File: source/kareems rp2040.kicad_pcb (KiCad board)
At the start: 2 copper layers, 29 x 57 mm, 38 parts, among them J1 USB_C_Receptacle_USB2.0_14P, J2 Conn_01x20, J3 Conn_01x20, J4 Conn_01x03, SW1 SW_Push, U1 RP2040, U2 W25Q16JVSS, U4 MCP1700x-330xxTT, Y1 12MHz

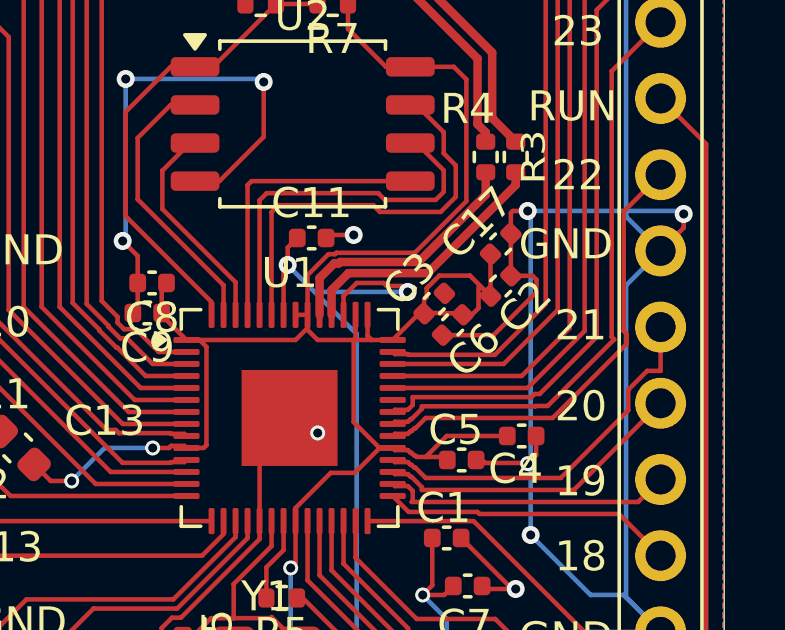
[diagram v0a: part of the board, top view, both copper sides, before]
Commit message: e
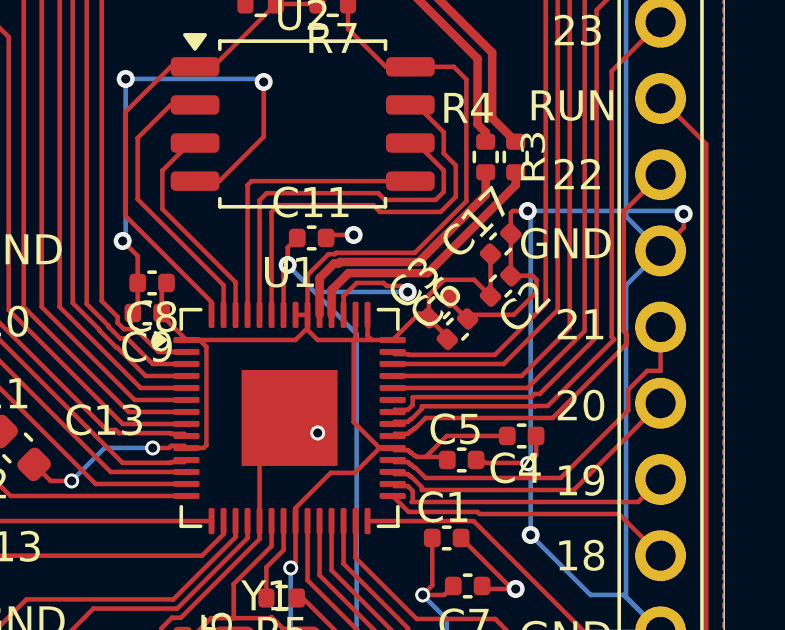
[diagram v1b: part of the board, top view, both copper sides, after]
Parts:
- moved C6 0.21 mm to (218.9, 100.3), turned to 45 degrees
- moved C3 0.21 mm to (218.2, 99.6)
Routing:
- net +3.3V: track 145.2 -> 143.3 mm
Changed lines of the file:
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@@
 	(footprint "Capacitor_SMD:C_0402_1005Metric"
 		(layer "F.Cu")
-		(at 218.7 100.2 -135)
+		(at 218.860589 100.339411 45)
 		(descr "Capacitor SMD 0402 (1005 Metric), square (rectangular) end terminal, IPC-7351 nominal, (Body size source: IPC-SM-782 page 76, https://www.pcb-3d.com/wordpress/wp-content/uploads/ipc-sm-782a_amendment_1_and_2.pdf), generated with kicad-footprint-generator")
 		(tags "capacitor")
@@
 		(attr smd)
 		(fp_line
-			(start -0.107836 0.36)
-			(end 0.107836 0.36)
+			(start -0.107836 -0.36)
+			(end 0.107836 -0.36)
 			(stroke
 				(width 0.12)
@@
 		)
 		(fp_line
-			(start -0.107836 -0.36)
-			(end 0.107836 -0.36)
+			(start -0.107836 0.36)
+			(end 0.107836 0.36)
 			(stroke
 				(width 0.12)
@@
 		)
 		(pad "1" smd roundrect
-			(at -0.48 0 225)
+			(at -0.48 0 45)
 			(size 0.56 0.62)
 			(layers "F.Cu" "F.Mask" "F.Paste")
@@
 		)
 		(pad "2" smd roundrect
-			(at 0.48 0 225)
+			(at 0.48 0 45)
 			(size 0.56 0.62)
 			(layers "F.Cu" "F.Mask" "F.Paste")
@@
 	(footprint "Capacitor_SMD:C_0402_1005Metric"
 		(layer "F.Cu")
-		(at 218.085786 99.485786 45)
+		(at 218.246375 99.625197 45)
 		(descr "Capacitor SMD 0402 (1005 Metric), square (rectangular) end terminal, IPC-7351 nominal, (Body size source: IPC-SM-782 page 76, https://www.pcb-3d.com/wordpress/wp-content/uploads/ipc-sm-782a_amendment_1_and_2.pdf), generated with kicad-footprint-generator")
 		(tags "capacitor")
@@
 	)
 	(segment
-		(start 220.060589 100.539411)
-		(end 221.4942 99.1058)
+		(start 211.4 110.85)
+		(end 213.1 112.55)
 		(width 0.1524)
 		(layer "F.Cu")
@@
 	)
 	(segment
-		(start 211.4 110.85)
-		(end 213.1 112.55)
+		(start 221.4942 98.6942)
+		(end 221.360589 98.560589)
 		(width 0.1524)
 		(layer "F.Cu")
@@
 	)
 	(segment
+		(start 219.039411 99.860589)
+		(end 220.739411 99.860589)
+		(width 0.1524)
+		(layer "F.Cu")
+		(net 1)
+	)
+	(segment
 		(start 212.2625 107.3375)
 		(end 209.641 109.959)
@@
 	)
 	(segment
-		(start 220.8 109)
-		(end 220.68 109)
+		(start 218.425197 99.146375)
+		(end 218.425197 99.246375)
 		(width 0.1524)
 		(layer "F.Cu")
@@
 	)
 	(segment
-		(start 218.360589 100.539411)
-		(end 220.060589 100.539411)
+		(start 220.8 109)
+		(end 220.68 109)
 		(width 0.1524)
 		(layer "F.Cu")
@@
 	)
 	(segment
+		(start 218.425197 99.246375)
+		(end 219.039411 99.860589)
+		(width 0.1524)
+		(layer "F.Cu")
+		(net 1)
+	)
+	(segment
 		(start 199.7904 101.0904)
 		(end 200.4304 101.7304)
@@
 	)
 	(segment
-		(start 221.4942 99.1058)
-		(end 221.4942 98.6942)
+		(start 216.8375 81.2375)
+		(end 215.325 79.725)
 		(width 0.1524)
 		(layer "F.Cu")
@@
 	)
 	(segment
-		(start 216.8375 81.2375)
-		(end 215.325 79.725)
+		(start 221.360589 98.560589)
+		(end 220.639411 98.560589)
 		(width 0.1524)
 		(layer "F.Cu")
@@
 	)
 	(segment
+		(start 220.739411 99.860589)
+		(end 221.4942 99.1058)
+		(width 0.1524)
+		(layer "F.Cu")
+		(net 1)
+	)
+	(segment
 		(start 210.35 110.85)
 		(end 209.7 111.5)
@@
 	)
 	(segment
-		(start 221.4942 98.6942)
-		(end 221.360589 98.560589)
+		(start 219.039411 99.860589)
+		(end 219.339411 99.860589)
 		(width 0.1524)
 		(layer "F.Cu")
@@
 	)
 	(segment
-		(start 221.360589 98.560589)
-		(end 220.639411 98.560589)
+		(start 221.4942 99.1058)
+		(end 221.4942 98.6942)
 		(width 0.1524)
 		(layer "F.Cu")
@@
 	)
 	(segment
-		(start 219.560589 99.639411)
-		(end 219.560589 98.939411)
-		(width 0.1524)
-		(layer "F.Cu")
-		(net 2)
-	)
-	(segment
 		(start 209.825 100.7)
 		(end 210.2625 100.7)
@@
 	)
 	(segment
-		(start 217.83365 98.974812)
-		(end 218.253634 98.554828)
-		(width 0.1524)
-		(layer "F.Cu")
-		(net 2)
-	)
-	(segment
-		(start 217.771572 99.8)
-		(end 218.257164 99.8)
-		(width 0.1524)
-		(layer "F.Cu")
-		(net 2)
-	)
-	(segment
 		(start 217.8 104.6)
 		(end 218.5 103.9)
@@
 	)
 	(segment
-		(start 218.257164 99.8)
-		(end 218.266486 99.809322)
-		(width 0.1524)
-		(layer "F.Cu")
-		(net 2)
-	)
-	(segment
 		(start 226.781 66.099)
 		(end 224.601 66.099)
@@
 	)
 	(segment
-		(start 218.988144 99.809322)
-		(end 219.039411 99.860589)
-		(width 0.1524)
-		(layer "F.Cu")
-		(net 2)
-	)
-	(segment
 		(start 213.4625 108.1375)
 		(end 213.3 108.3)
@@
 	)
 	(segment
-		(start 219.276006 98.554828)
-		(end 219.960589 99.239411)
-		(width 0.1524)
-		(layer "F.Cu")
-		(net 2)
-	)
-	(segment
 		(start 213.8625 100.3)
 		(end 213.4625 100.7)
@@
 	)
 	(segment
-		(start 218.5 103.9)
-		(end 220.52 103.9)
-		(width 0.1524)
-		(layer "F.Cu")
-		(net 2)
-	)
-	(segment
-		(start 213.4625 106.7375)
-		(end 213.4625 108.1375)
+		(start 218.360589 100.539411)
+		(end 218.360589 100.439411)
 		(width 0.1524)
 		(layer "F.Cu")
@@
 	)
 	(segment
-		(start 217.2875 91.595)
-		(end 216.475001 91.595)
+		(start 218.414223 98.694239)
+		(end 219.415417 98.694239)
 		(width 0.1524)
 		(layer "F.Cu")
@@
 	)
 	(segment
-		(start 219.58 71.12)
-		(end 218.28 71.12)
+		(start 218.5 103.9)
+		(end 220.52 103.9)
 		(width 0.1524)
 		(layer "F.Cu")
@@
 	)
 	(segment
-		(start 217.746375 99.825197)
-		(end 217.746375 99.353625)
+		(start 213.4625 106.7375)
+		(end 213.4625 108.1375)
 		(width 0.1524)
 		(layer "F.Cu")
@@
 	)
 	(segment
-		(start 217.746375 99.353625)
-		(end 217.83365 99.26635)
+		(start 217.2875 91.595)
+		(end 216.475001 91.595)
 		(width 0.1524)
 		(layer "F.Cu")
@@
 	)
 	(segment
-		(start 218.253634 98.554828)
-		(end 219.276006 98.554828)
+		(start 219.58 71.12)
+		(end 218.28 71.12)
 		(width 0.1524)
 		(layer "F.Cu")
@@
 	)
 	(segment
-		(start 217.83365 99.26635)
-		(end 217.83365 98.974812)
+		(start 210.2625 100.7)
+		(end 210.4921 100.9296)
 		(width 0.1524)
 		(layer "F.Cu")
@@
 	)
 	(segment
-		(start 210.2625 100.7)
-		(end 210.4921 100.9296)
+		(start 213.8625 100.364116)
+		(end 214.198384 100.7)
 		(width 0.1524)
 		(layer "F.Cu")
@@
 	)
 	(segment
-		(start 213.8625 100.364116)
-		(end 214.198384 100.7)
+		(start 219.415417 98.694239)
+		(end 219.960589 99.239411)
 		(width 0.1524)
 		(layer "F.Cu")
@@
 	)
 	(segment
+		(start 218.360589 100.439411)
+		(end 217.746375 99.825197)
+		(width 0.1524)
+		(layer "F.Cu")
+		(net 2)
+	)
+	(segment
 		(start 213.4625 99.8625)
 		(end 213.8625 99.8625)
@@
 	)
 	(segment
-		(start 215.21 87.529596)
-		(end 215.21 89.5)
+		(start 217.906964 99.201498)
+		(end 218.414223 98.694239)
 		(width 0.1524)
 		(layer "F.Cu")
@@
 	)
 	(segment
-		(start 207.9 79.047583)
-		(end 209.5625 80.710083)
+		(start 217.906964 99.964608)
+		(end 217.906964 99.201498)
 		(width 0.1524)
 		(layer "F.Cu")
@@
 	)
 	(segment
-		(start 219.339411 99.860589)
-		(end 219.560589 99.639411)
+		(start 215.21 87.529596)
+		(end 215.21 89.5)
+		(width 0.1524)
+		(layer "F.Cu")
+		(net 2)
+	)
+	(segment
+		(start 207.9 79.047583)
+		(end 209.5625 80.710083)
 		(width 0.1524)
 		(layer "F.Cu")
@@
 	)
 	(segment
-		(start 218.266486 99.809322)
-		(end 218.988144 99.809322)
-		(width 0.1524)
-		(layer "F.Cu")
-		(net 2)
-	)
-	(segment
 		(start 209.3203 104.2296)
 		(end 209.2499 104.3)
@@
 		(width 0.1524)
 		(layer "F.Cu")
-		(net 2)
-	)
-	(segment
-		(start 219.039411 99.860589)
-		(end 219.339411 99.860589)
-		(width 0.1524)
-		(layer "F.Cu")

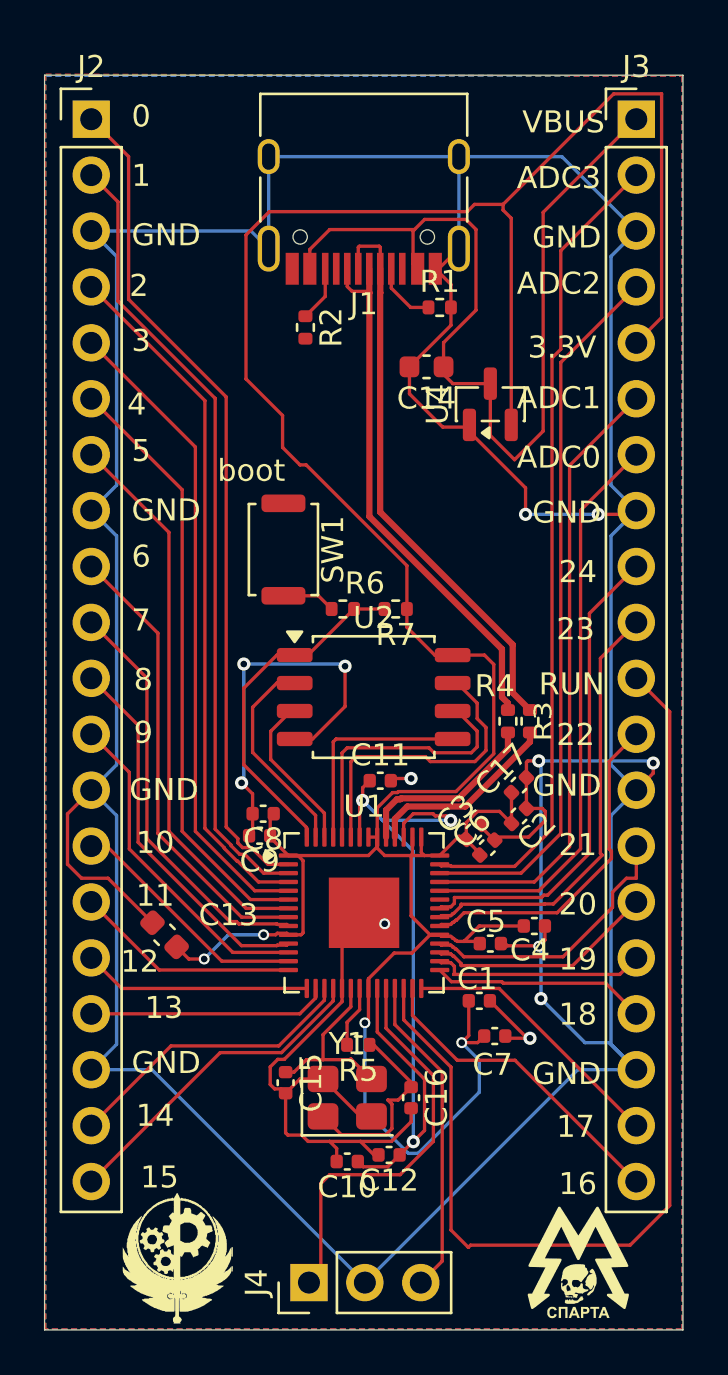
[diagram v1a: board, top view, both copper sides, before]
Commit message: ee
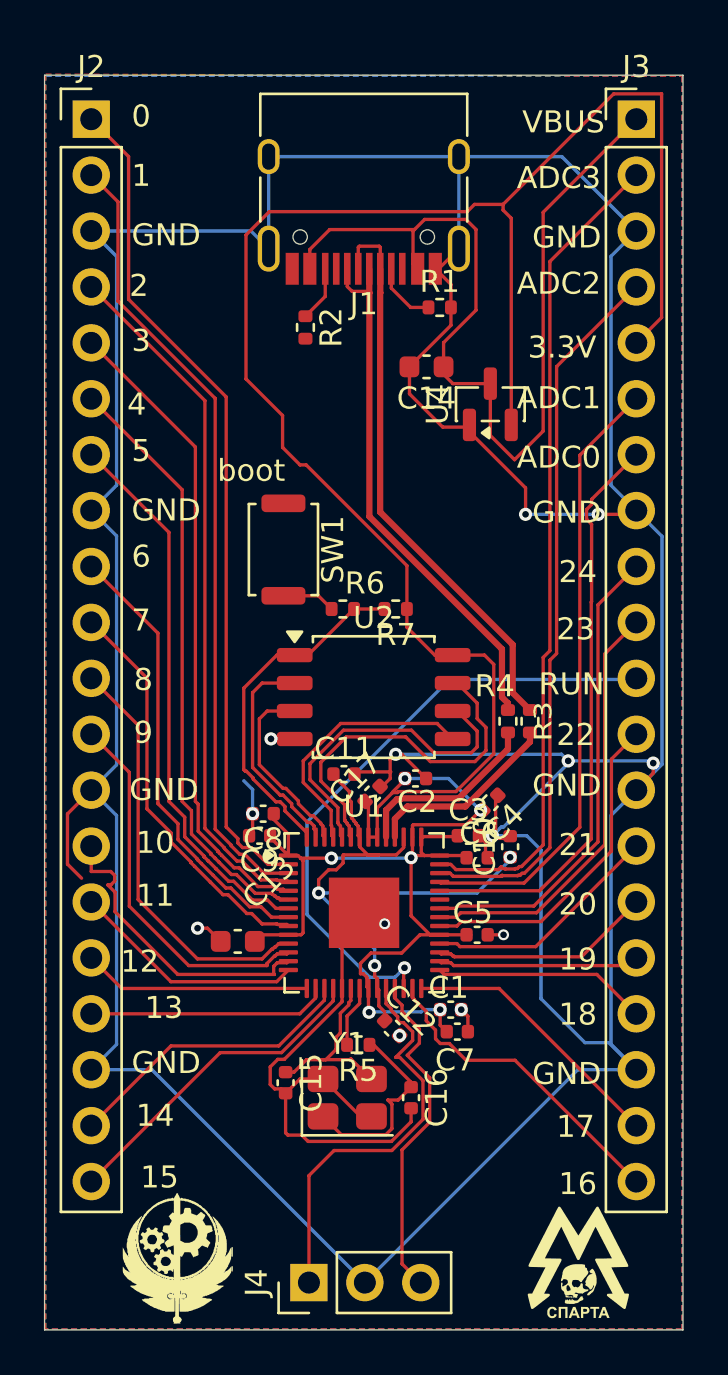
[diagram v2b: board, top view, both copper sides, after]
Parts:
- moved C10 16.1 mm to (219.9, 100.3), turned to 90 degrees
- moved C17 6.66 mm to (213.7, 97.9)
- moved C4 5.95 mm to (219.0, 98.3), turned to 45 degrees
- moved C12 5.76 mm to (214.5, 108.5), turned to -45 degrees
- moved C2 5.00 mm to (215.6, 97.2), turned to 0 degrees
- moved C13 3.34 mm to (207.5, 104.6), turned to 180 degrees
- moved C7 1.71 mm to (217.5, 108.7)
- moved C11 1.68 mm to (212.3, 97.0)
- moved C1 1.36 mm to (217.2, 107.7)
- moved C5 0.72 mm to (218.4, 104.3)
- moved C6 0.65 mm to (218.4, 100.8), turned to 0 degrees
- moved C3 0.30 mm to (218.0, 99.8), turned to 0 degrees
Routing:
- net RUN: track 47.5 -> 28.6 mm, vias 0 -> 1
- net +3.3V: track 143.3 -> 129.4 mm, vias 4 -> 6
- net GND: track 262.5 -> 249.8 mm, vias 12 -> 13
- net +1V1: track 36.5 -> 26.5 mm
- net GPIO10: track 11.1 -> 13.9 mm
- net QSPI_SD3: track 13.8 -> 16.4 mm
- net QSPI_SCLK: track 12.5 -> 14.9 mm
- net GPIO9: track 15.1 -> 17.2 mm
- net GPIO8: track 17.1 -> 19.2 mm
- net QSPI_SD0: track 9.80 -> 11.8 mm
- net GPIO21: track 12.5 -> 10.9 mm
- net QSPI_SD2: track 7.29 -> 8.50 mm
- net SWD: track 14.7 -> 15.4 mm
- net GPIO19: track 9.75 -> 9.16 mm
- net QSPI_SD1: track 9.45 -> 10.00 mm
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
